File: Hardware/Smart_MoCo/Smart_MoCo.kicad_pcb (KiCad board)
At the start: 4 copper layers, 33.4 x 42.3 mm, 32 parts, among them J1 Conn_01x04, J2 1722861102, J4 1722861102, U1 STM32F042F6Px, U2 VNH5019A-E, U3 SN65HVD232, U4 AP62200WU

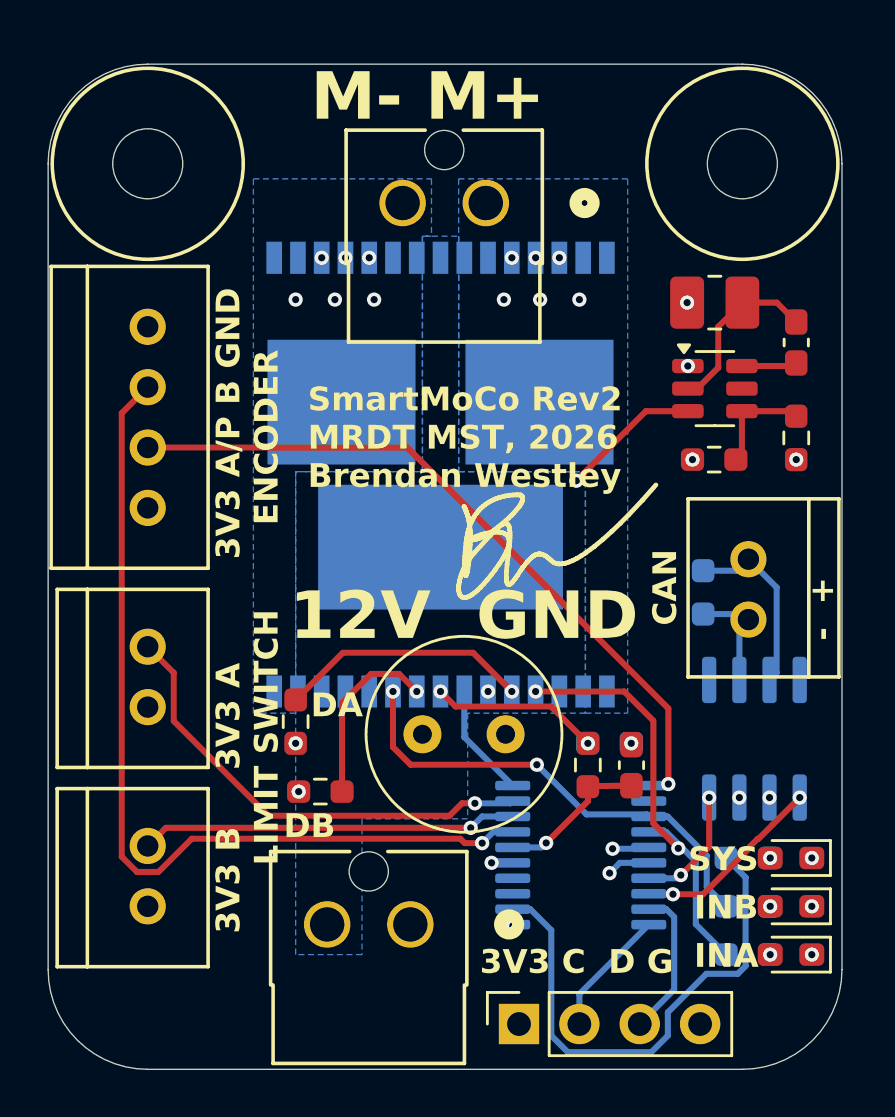
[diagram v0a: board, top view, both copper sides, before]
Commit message: Melt traces
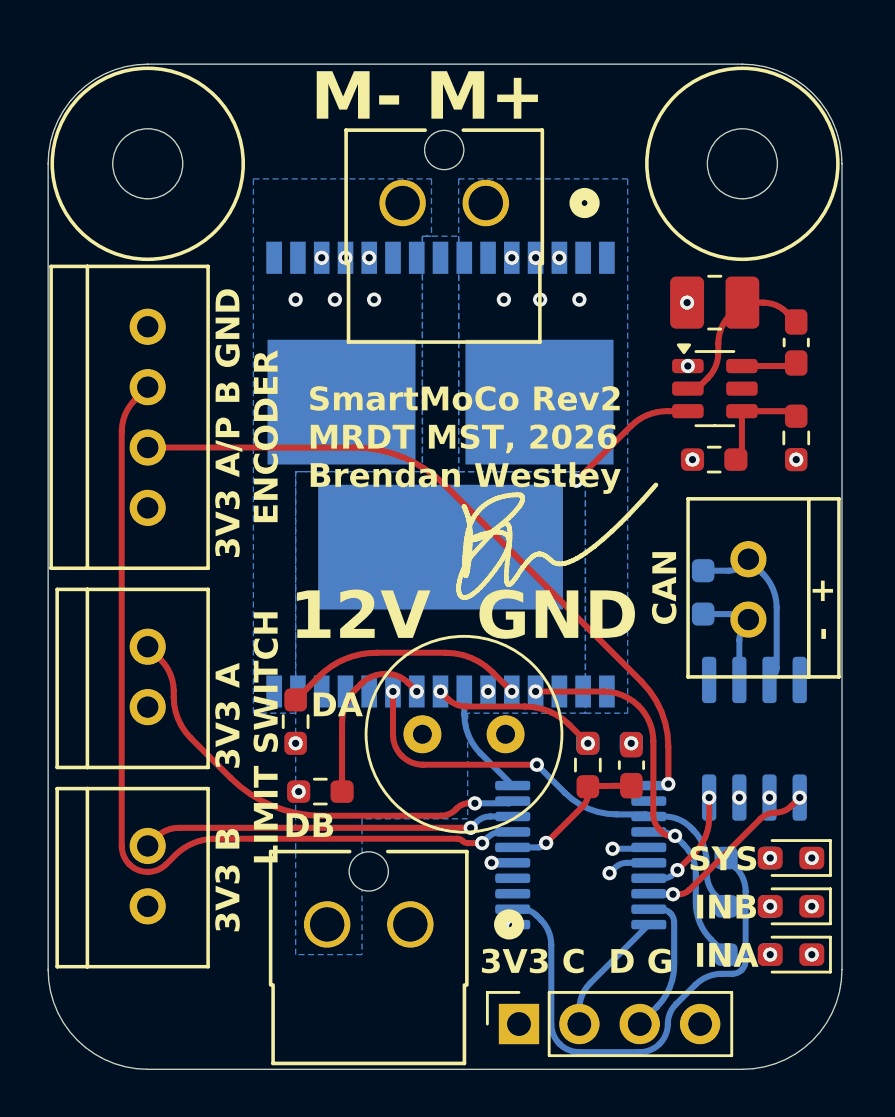
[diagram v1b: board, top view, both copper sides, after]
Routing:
- net IN_A: track 18.2 -> 17.5 mm
- net LED_STATUS: track 21.8 -> 21.2 mm
- net LIM_B: track 19.7 -> 19.2 mm
